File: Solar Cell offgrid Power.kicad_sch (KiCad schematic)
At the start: 12 parts, among them J1 Conn_01x10_Socket, J2 Conn_01x10_Pin, J3 Screw_Terminal_01x02, Q1 S8550

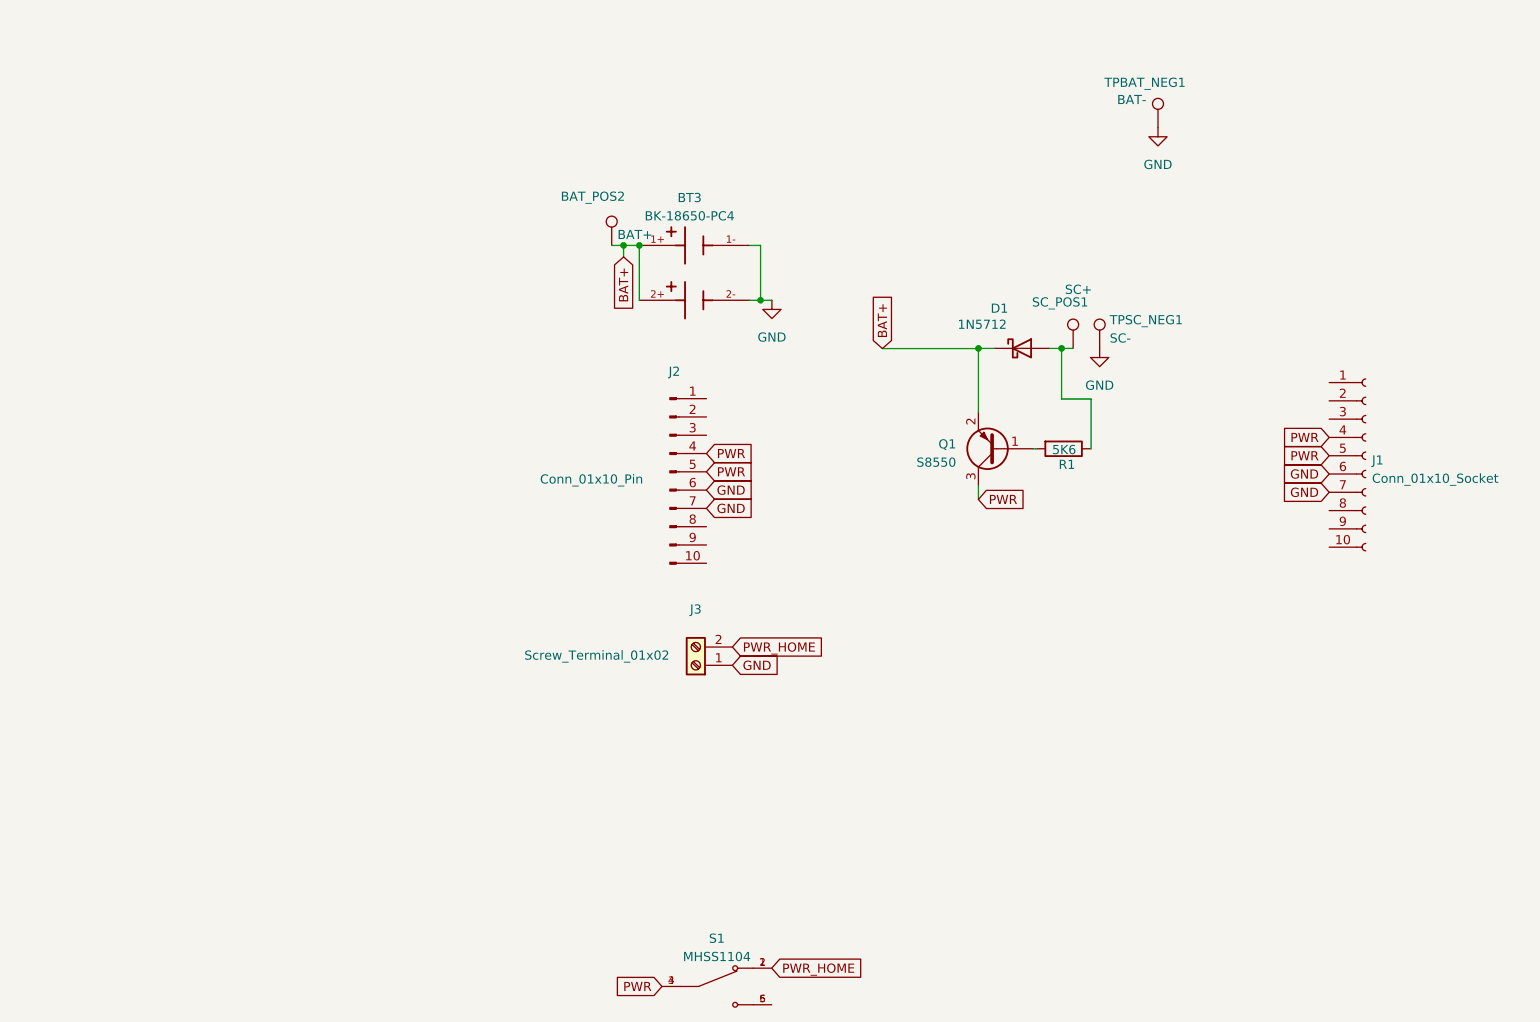
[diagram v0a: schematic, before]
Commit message: Add files via upload
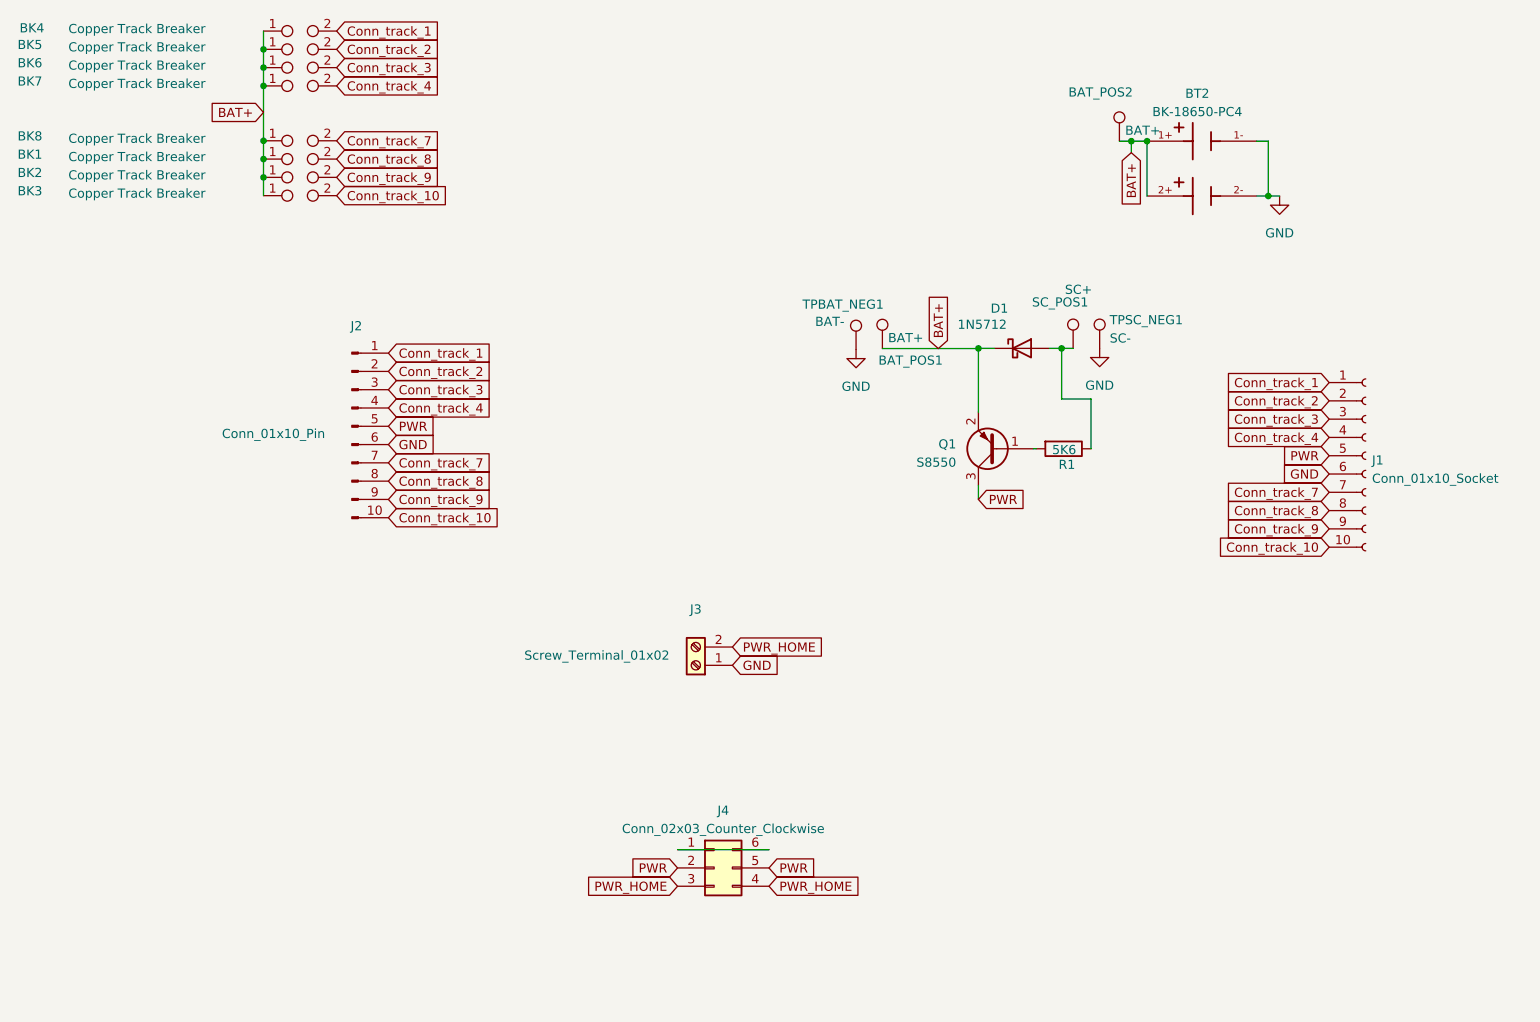
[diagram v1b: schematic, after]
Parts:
- removed BT3: BK-18650-PC4, Battery:2x 18650 Battery holder BAT_BK-18650-PC4, symbol Connector:2x_18650_battery_holder_BK-18650-PC4
- removed S1: MHSS1104, Button_Switch_THT:Toggle Switch 2 pos PCB MSS-22D18G2 2P2T, symbol Switch:toggle_switch_2_pos__SOT_SMD_MHSS1104
- added BAT_POS1: BAT+, TestPoint:TestPoint_Pad_3.0x3.0mm, symbol Connector:TestPoint
- added BK1, BK2, BK3, BK4, BK5, BK6, BK7, BK8: Copper Track Breaker, AeonLabs_Connectors:Copper Track Breaker 2 points, symbol AeonLabs_Connectors:Copper_Track_Break_2_points
- added BT2: BK-18650-PC4, Battery:2x 18650 Battery holder BAT_BK-18650-PC4, symbol Connector:2x_18650_battery_holder_BK-18650-PC4
- added J4: Conn_02x03_Counter_Clockwise, Button_Switch_THT:Toggle Switch 2 pos PCB MSS-22D18G2 2P2T, symbol Connector_Generic:Conn_02x03_Counter_Clockwise
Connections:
- net BAT+: now also BAT_POS1.1, BK1.1, BK2.1, BK3.1, BK4.1, BK5.1, BK6.1, BK7.1, BK8.1, BT2.1+, BT2.2+
- net GND: now also BT2.1-, BT2.2-; no longer J1.7 (Pin_7), J2.7 (Pin_7)
- net PWR: now also J4.2 (Pin_2), J4.5 (Pin_5); no longer J1.4 (Pin_4), J2.4 (Pin_4)
- net PWR_HOME: now also J4.3 (Pin_3), J4.4 (Pin_4)
- net Conn_track_1: now reaches J2.1 (Pin_1)
- net Conn_track_1: now also J1.1 (Pin_1), BK4.2
- net Conn_track_10: now reaches J2.10 (Pin_10)
- net Conn_track_10: now also J1.10 (Pin_10), BK3.2
- net Conn_track_2: now reaches J2.2 (Pin_2)
- net Conn_track_2: now also J1.2 (Pin_2), BK5.2
- net Conn_track_3: now reaches J2.3 (Pin_3)
- net Conn_track_3: now also J1.3 (Pin_3), BK6.2
- net Conn_track_8: now reaches J2.8 (Pin_8)
- net Conn_track_8: now also J1.8 (Pin_8), BK1.2
- net Conn_track_9: now reaches J2.9 (Pin_9)
- net Conn_track_9: now also J1.9 (Pin_9), BK2.2
- new net: J4.1 (Pin_1), J4.6 (Pin_6)
- new net Conn_track_4: BK7.2, J1.4 (Pin_4), J2.4 (Pin_4)
- new net Conn_track_7: BK8.2, J1.7 (Pin_7), J2.7 (Pin_7)
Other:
- moved on the sheet: J2, TPBAT_NEG1
